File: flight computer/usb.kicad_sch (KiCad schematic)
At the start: 33 parts, among them J11 USB_C_Receptacle_USB2.0_16P, J23 USB_C_Receptacle_USB2.0_16P, J24 USB_C_Receptacle_USB2.0_16P

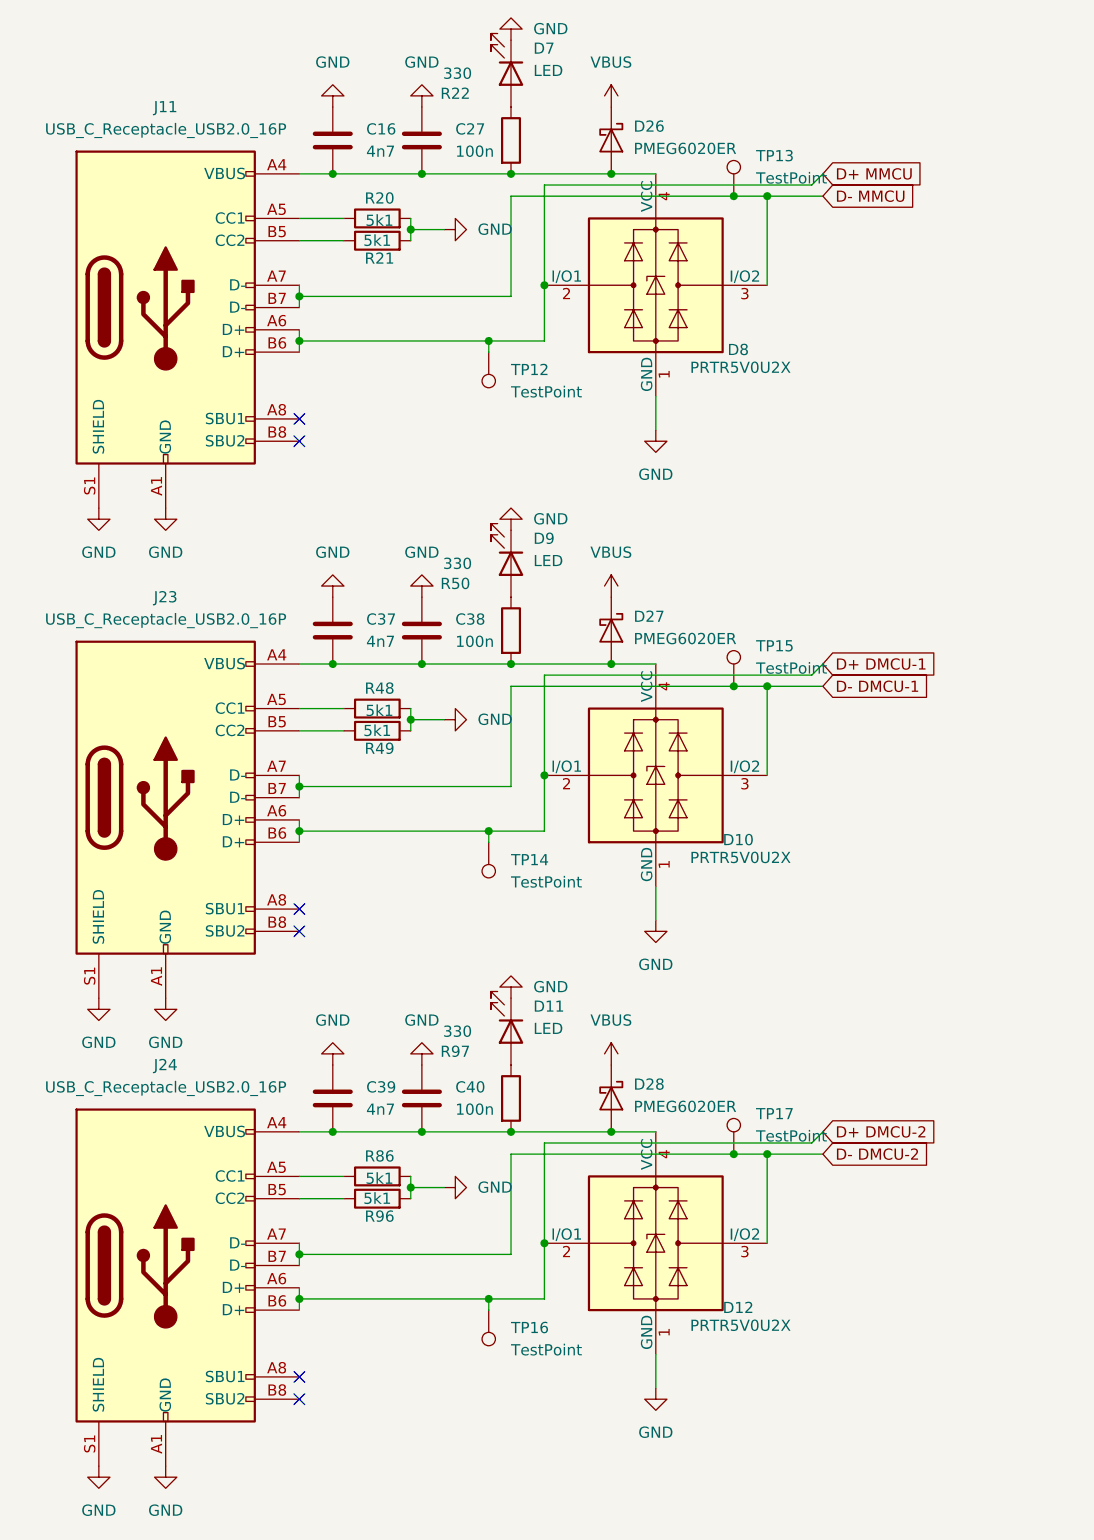
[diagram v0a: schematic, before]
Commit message: tspmo
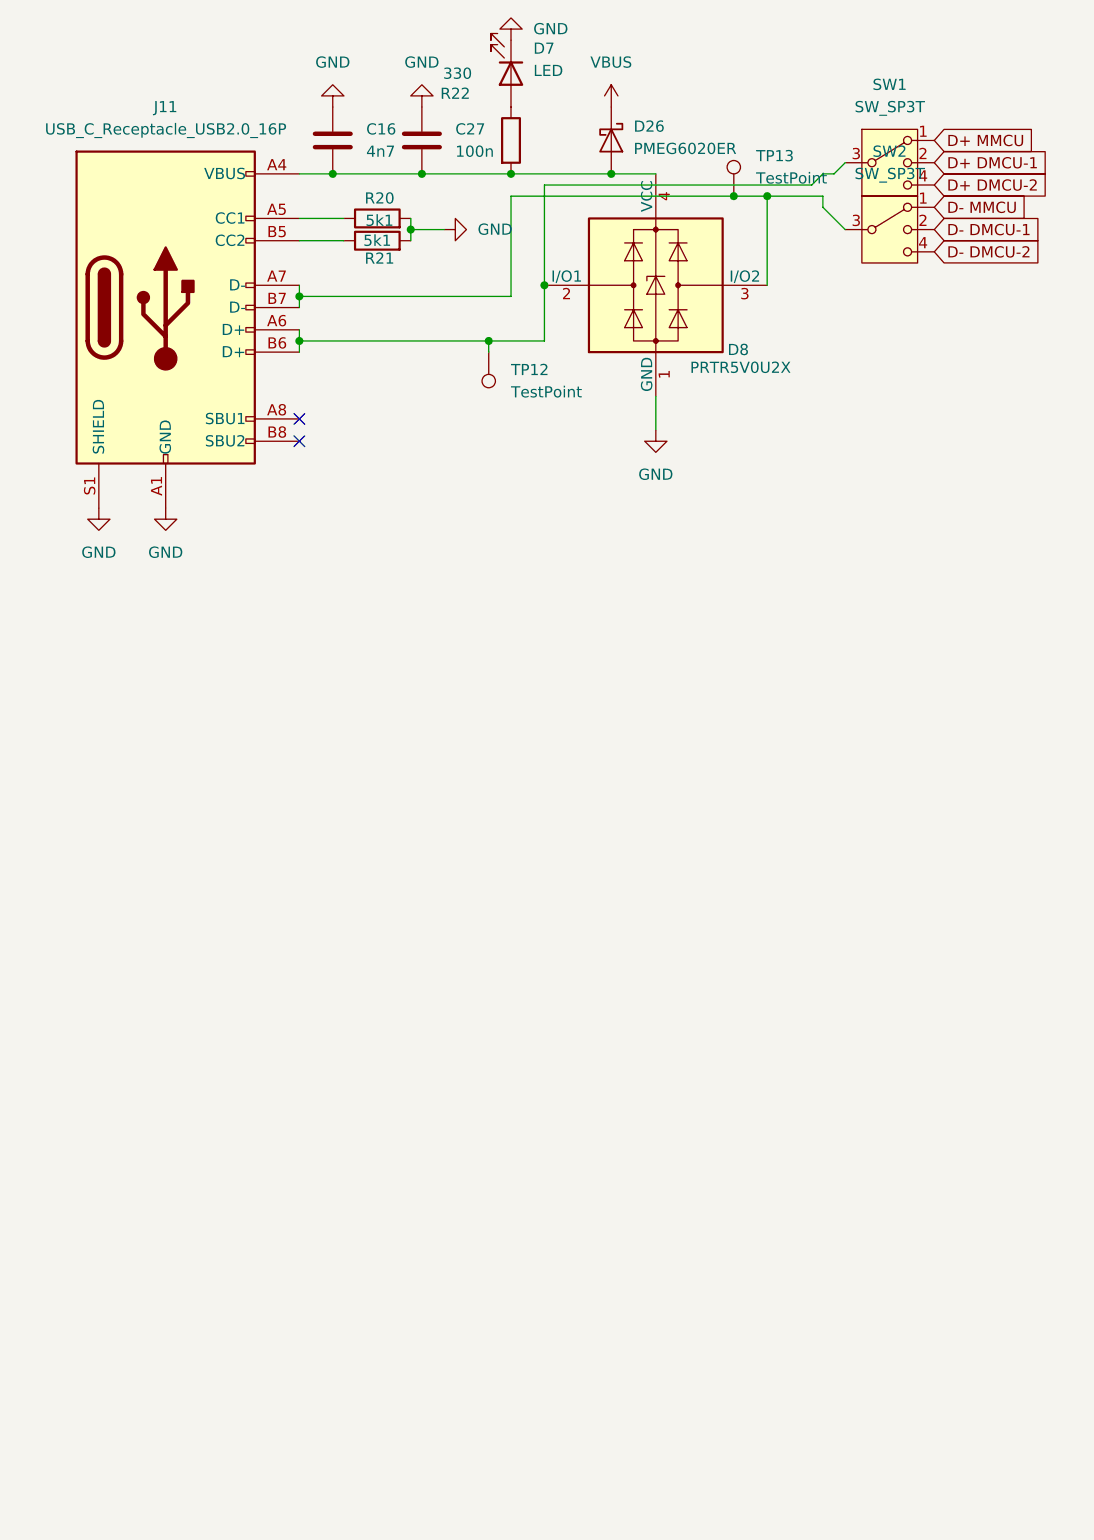
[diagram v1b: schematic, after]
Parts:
- removed C37, C39: 4n7, Capacitor_SMD:C_0603_1608Metric, symbol Device:C
- removed C38, C40: 100n, Capacitor_SMD:C_0603_1608Metric, symbol Device:C
- removed D10, D12: PRTR5V0U2X, Package_TO_SOT_SMD:SOT-143, symbol Power_Protection:PRTR5V0U2X
- removed D11, D9: LED, LED_SMD:LED_0603_1608Metric, symbol Device:LED
- removed D27, D28: PMEG6020ER, Diode_SMD:Nexperia_CFP3_SOD-123W, symbol Diode:PMEG6020ER
- removed J23, J24: USB_C_Receptacle_USB2.0_16P, Connector_USB:USB_C_Receptacle_GCT_USB4105-xx-A_16P_TopMnt_Horizontal, symbol Connector:USB_C_Receptacle_USB2.0_16P
- removed R48, R49, R86, R96: 5k1, Resistor_SMD:R_0603_1608Metric, symbol Device:R
- removed R50, R97: 330, Resistor_SMD:R_0603_1608Metric, symbol Device:R
- removed TP14, TP15, TP16, TP17: TestPoint, TestPoint:TestPoint_Pad_1.0x1.0mm, symbol Connector:TestPoint
- added SW1, SW2: SW_SP3T, NR01103ANG13-1C:SW_NR01103ANG13-1C, symbol Switch:SW_SP3T
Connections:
- net D+ DMCU-1: now also SW1.2
- net D+ DMCU-2: now also SW1.4
- net D+ MMCU: now also SW1.1; no longer D8.2 (I/O1), J11.A6 (D+), J11.B6 (D+), TP12.1
- net D- DMCU-1: now also SW2.2
- net D- DMCU-2: now also SW2.4
- net D- MMCU: now also SW2.1; no longer D8.3 (I/O2), J11.A7 (D-), J11.B7 (D-), TP13.1
- new net: D8.3 (I/O2), J11.A7 (D-), J11.B7 (D-), SW2.3, TP13.1
- new net: D8.2 (I/O1), J11.A6 (D+), J11.B6 (D+), SW1.3, TP12.1
- no-connect marks 6 -> 2
